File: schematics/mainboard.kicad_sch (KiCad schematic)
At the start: 5 parts

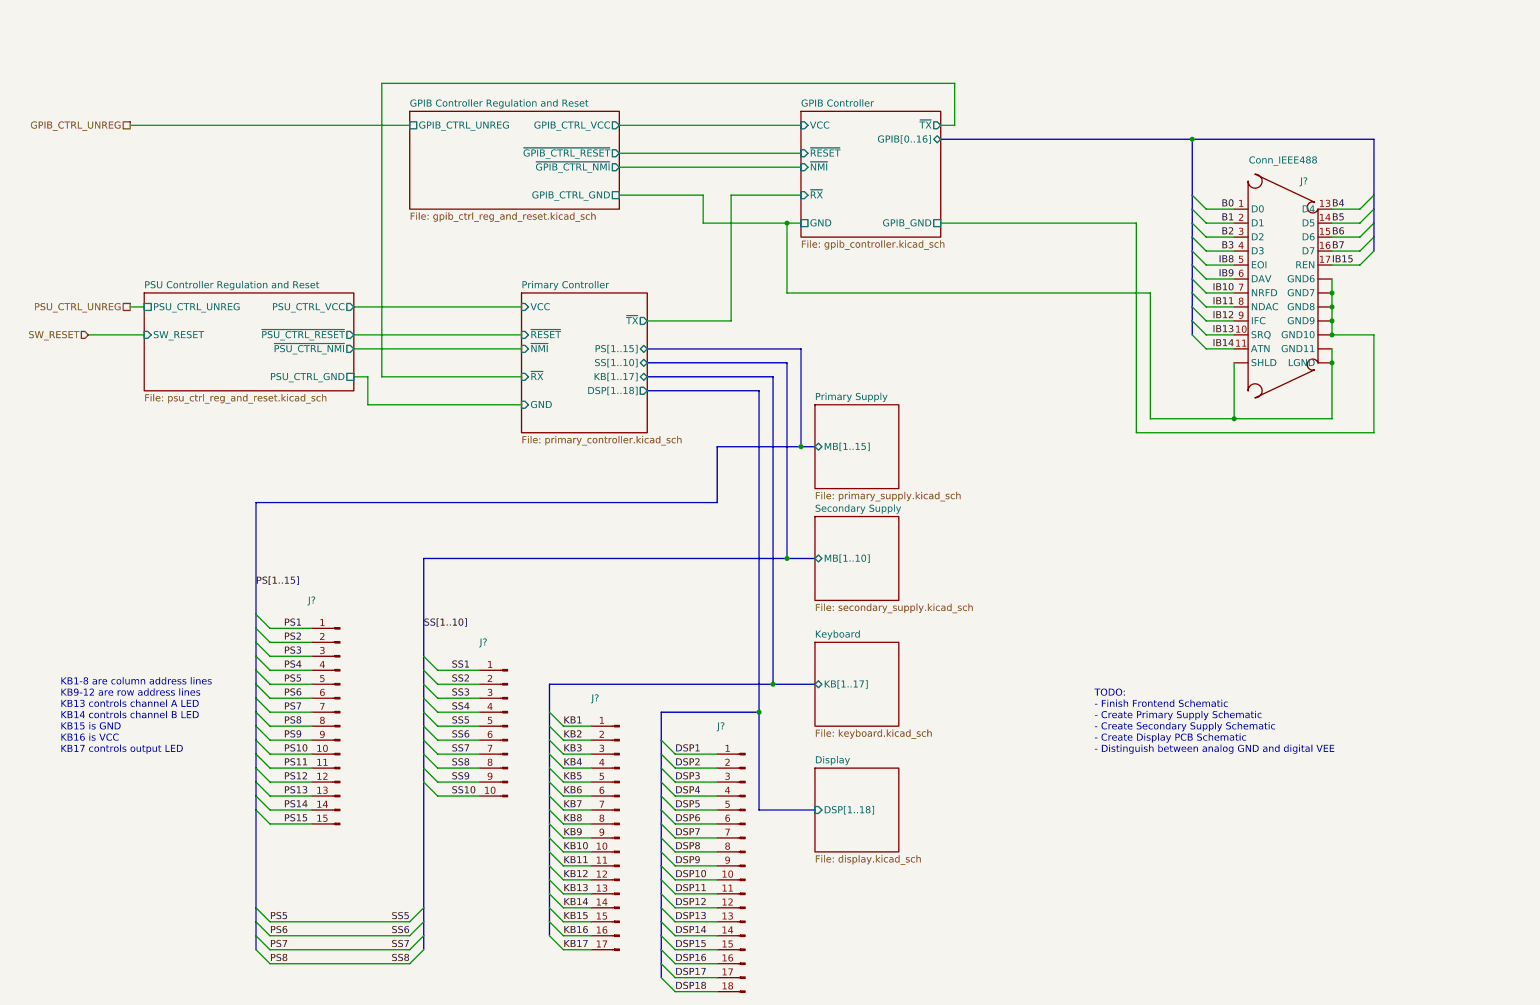
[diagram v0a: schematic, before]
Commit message: cleanup, fixes, started on power supplies
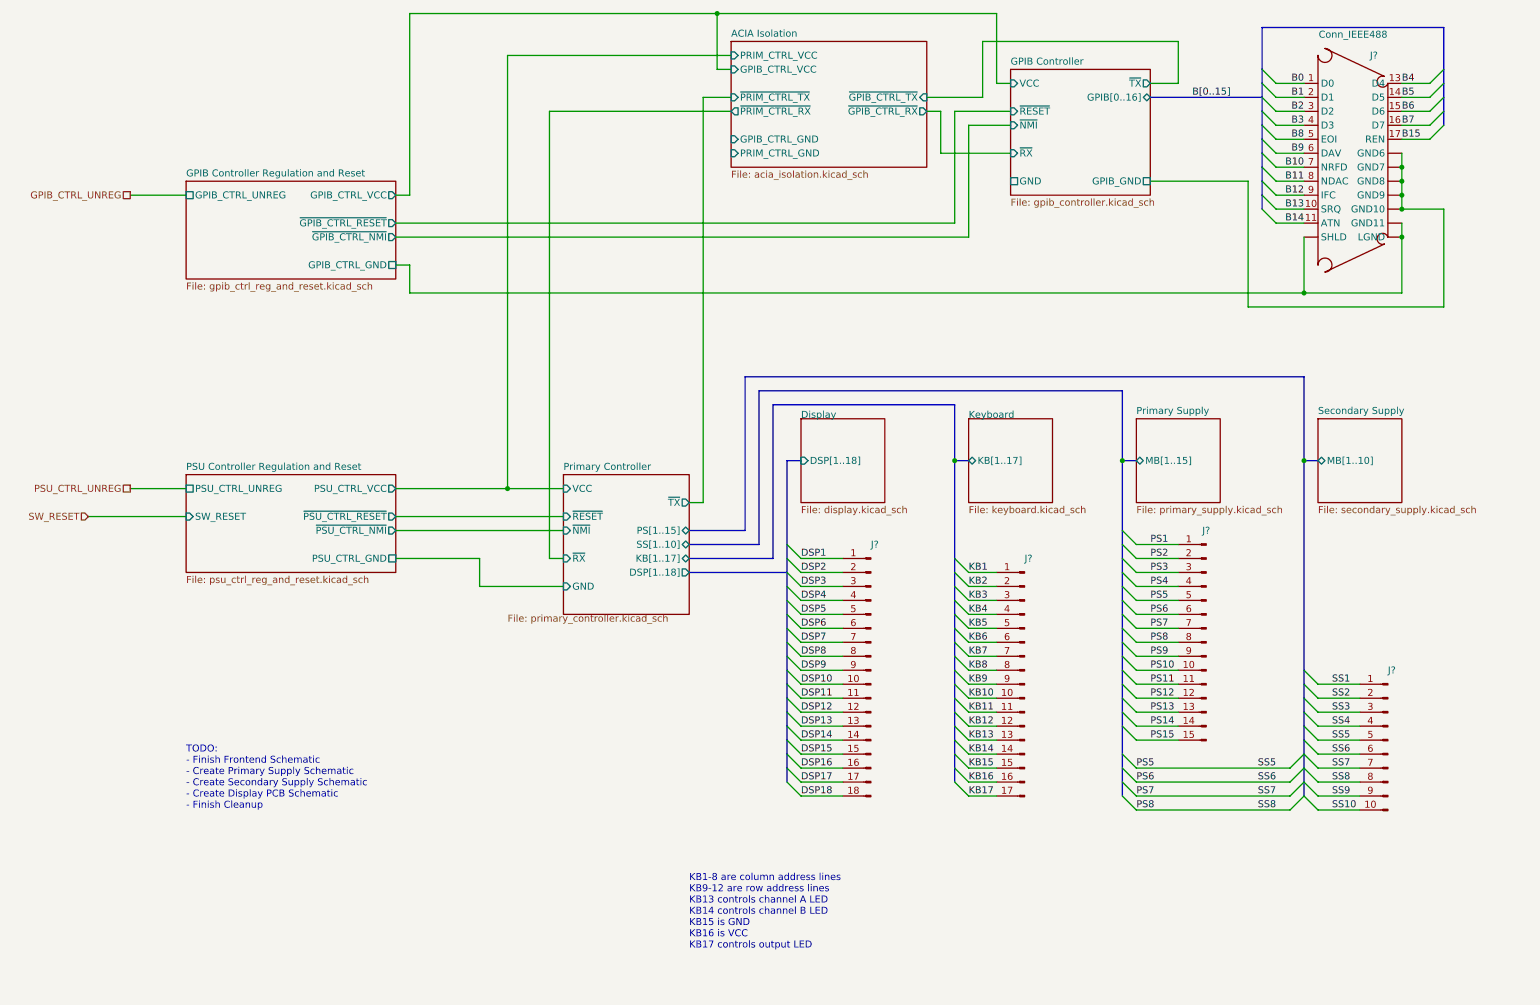
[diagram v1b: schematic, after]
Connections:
- net IB10 renamed B10
- net IB11 renamed B11
- net IB12 renamed B12
- net IB13 renamed B13
- net IB14 renamed B14
- net IB15 renamed B15
- net IB8 renamed B8
- net IB9 renamed B9
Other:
- added sheet ACIA Isolation (acia_isolation.kicad_sch)
- note added: "TODO: - Finish Frontend Schematic - Create Primary Supply Schematic - Create Secondary Supply Schematic - Create Display PCB Schematic - Finish Cleanup"
- note removed: "TODO: - Finish Frontend Schematic - Create Primary Supply Schematic - Create Secondary Supply Schematic - Create Display PCB Schematic - Distinguish between analog GND and digital VEE"
- moved on the sheet: J?
